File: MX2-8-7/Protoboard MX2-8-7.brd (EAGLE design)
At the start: 64.4 x 71.2 mm, 137 parts, among them J1 DCJ0202

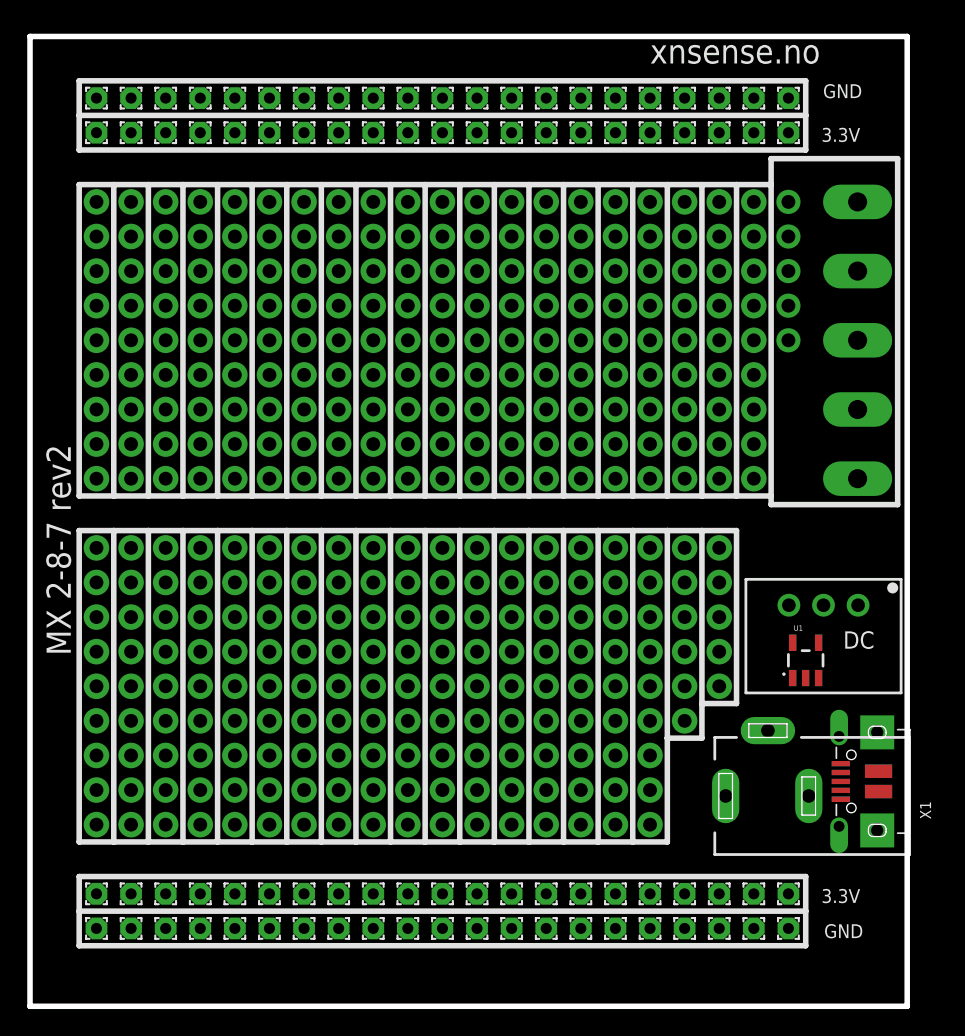
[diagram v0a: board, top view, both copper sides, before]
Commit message: Routed
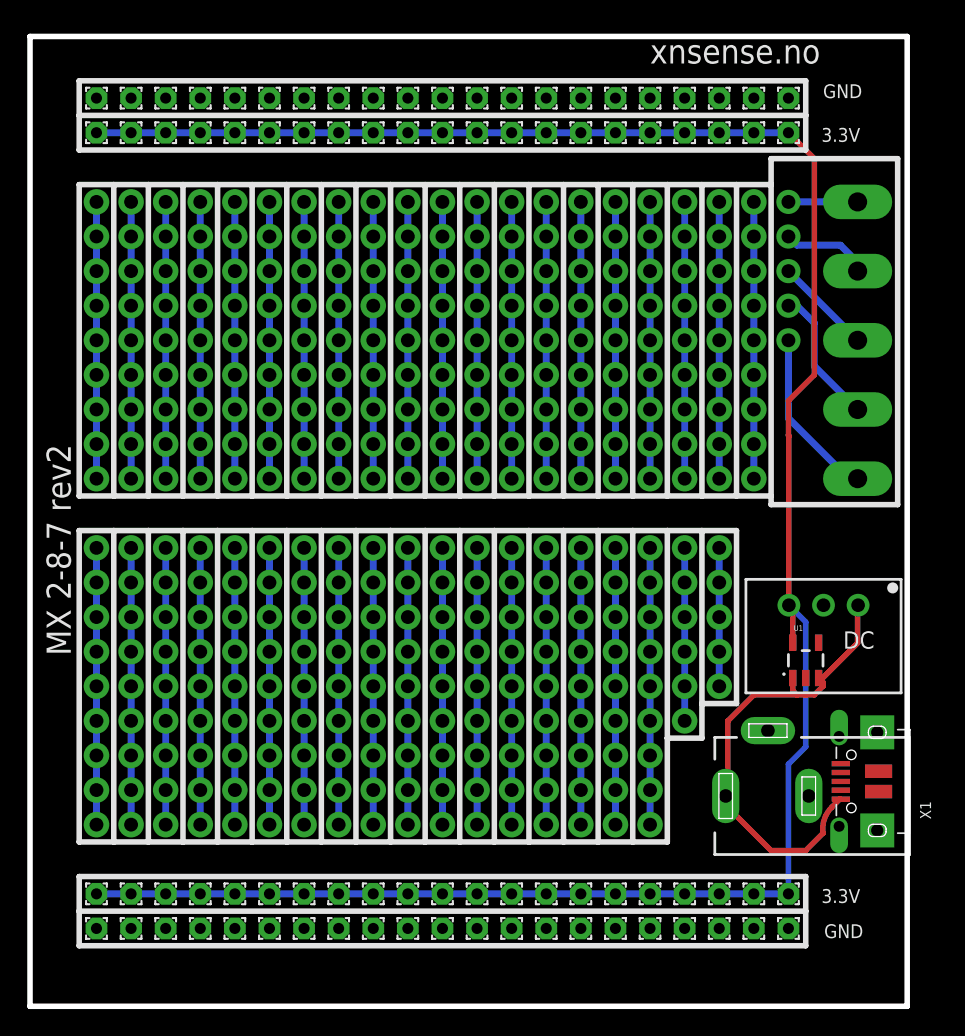
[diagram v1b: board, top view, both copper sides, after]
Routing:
- net VDD: track 0.00 -> 163.0 mm
- net VCC: track 0.00 -> 35.7 mm
- net N$9: track 0.00 -> 20.3 mm
- net N$8: track 0.00 -> 20.3 mm
- net N$7: track 0.00 -> 20.3 mm
- net N$6: track 0.00 -> 20.3 mm
- net N$5: track 0.00 -> 20.3 mm
- net N$4: track 0.00 -> 20.3 mm
- net N$39: track 0.00 -> 20.3 mm
- net N$38: track 0.00 -> 20.3 mm
- net N$37: track 0.00 -> 20.3 mm
- net N$36: track 0.00 -> 20.3 mm
- net N$35: track 0.00 -> 20.3 mm
- net N$33: track 0.00 -> 20.3 mm
- net N$32: track 0.00 -> 20.3 mm
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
